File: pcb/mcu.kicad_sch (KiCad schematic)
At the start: 38 parts, among them J1 CON_SAMTEC_14P_2R_1m27_P_KEY_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, U3 IC_MCU_STM32F100C4T6B_48LQFP, X1 XTAL_8M_20PPM_18pF_ECS-80-18-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, X2 XTAL_32K768_10PPM_7pF_ECS-.32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

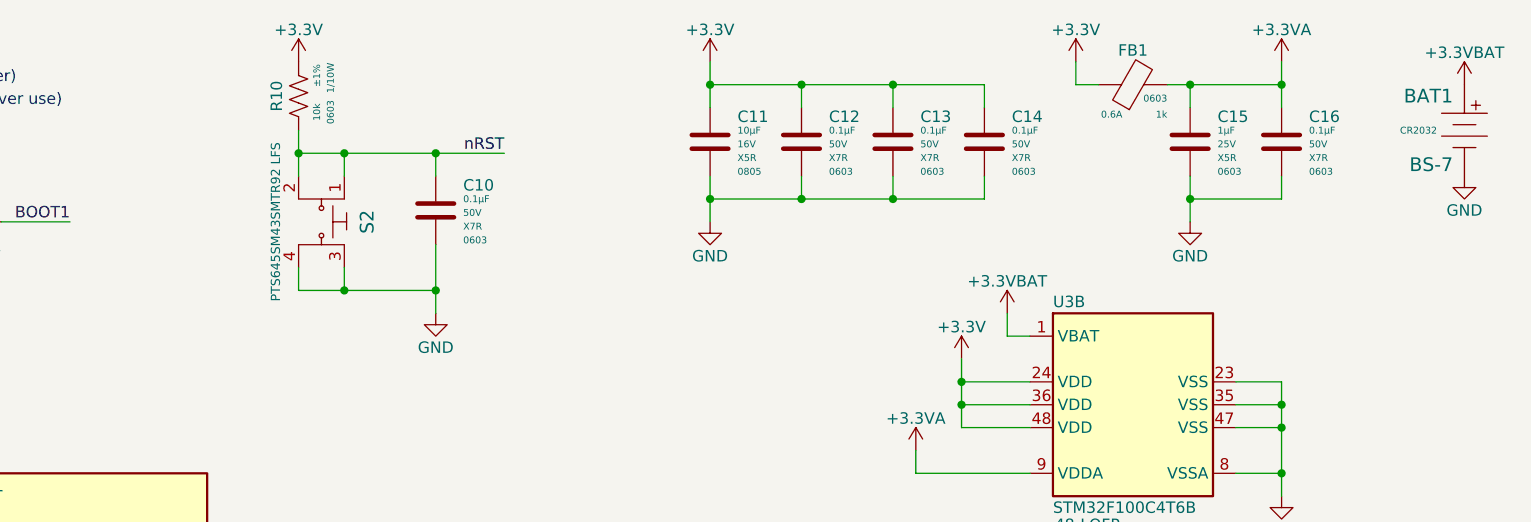
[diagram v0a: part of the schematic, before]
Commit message: Started mcu placement
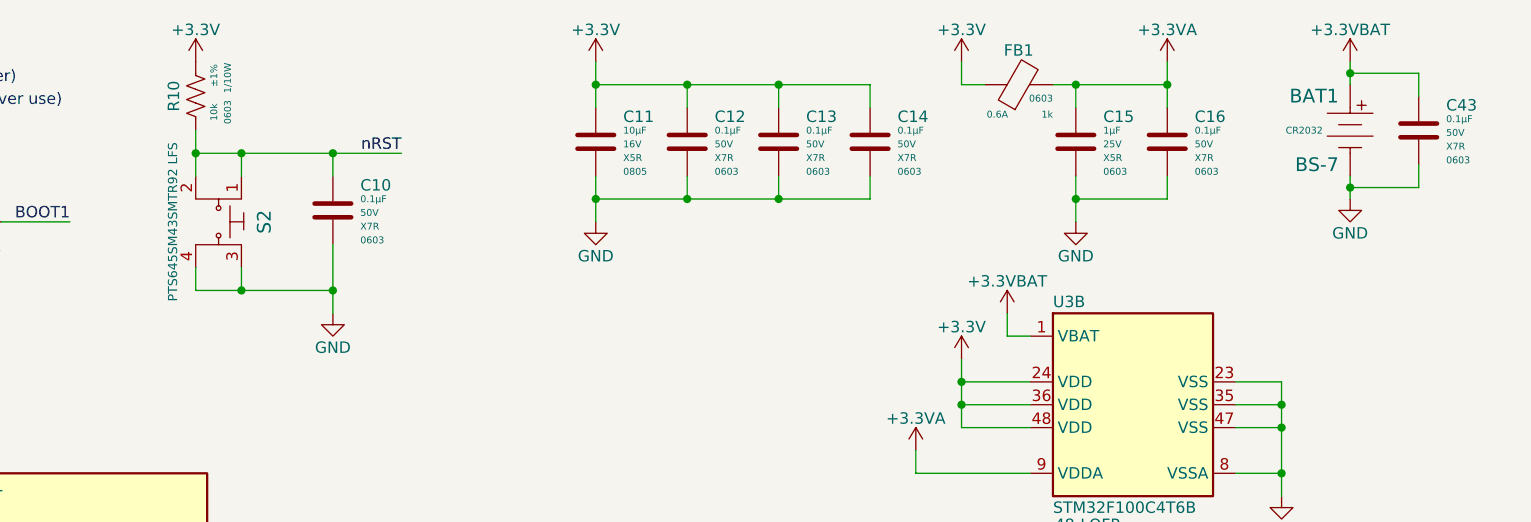
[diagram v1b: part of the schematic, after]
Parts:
- added C43: CAP_CER_0u1_50V_X7R_0603, Capacitor_SMD:C_0603_1608Metric, symbol arjun_symbols:CAP_CER_0u1_50V_X7R_0603
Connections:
- net +3.3VBAT: now also C43.1
- net GND: now also C43.2
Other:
- moved on the sheet: BAT1, C10, C11, C12, C13, C14, C15, C16, FB1, R10, S2
